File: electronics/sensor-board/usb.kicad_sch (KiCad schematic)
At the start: 6 parts, among them J16 USB_C_Receptacle_USB2.0

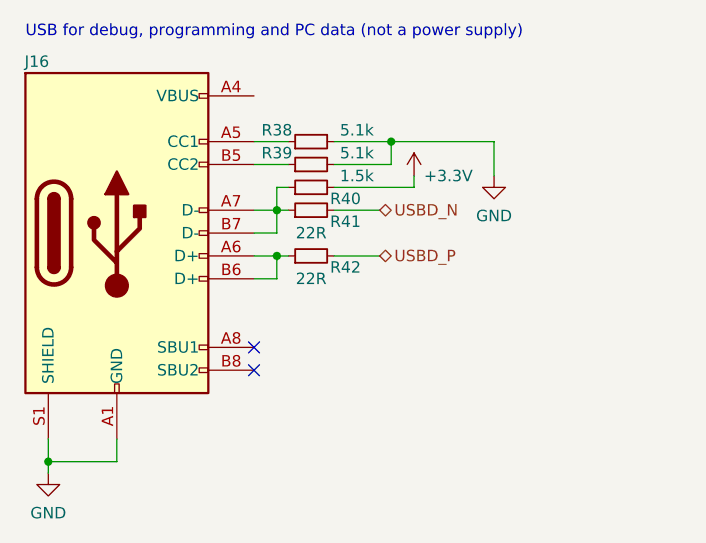
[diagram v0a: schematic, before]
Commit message: Further PCB layout
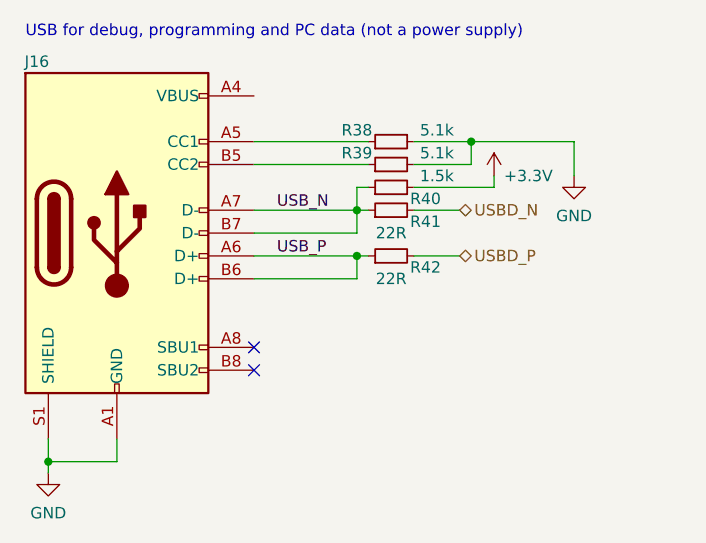
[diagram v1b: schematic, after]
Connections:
- net USB_N: now reaches J16.A7 (D-), J16.B7 (D-), R40.1, R41.1
- net USB_P: now reaches J16.A6 (D+), J16.B6 (D+), R42.1
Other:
- moved on the sheet: R38, R39, R40, R41, R42
